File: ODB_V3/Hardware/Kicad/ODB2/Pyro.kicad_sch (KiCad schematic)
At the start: 51 parts, among them J1 Screw_Terminal_01x08, U11 SI5442DU-T1-GE3, U12 SI5442DU-T1-GE3, U2 LM339, U3 SI5442DU-T1-GE3, U8 SI5442DU-T1-GE3

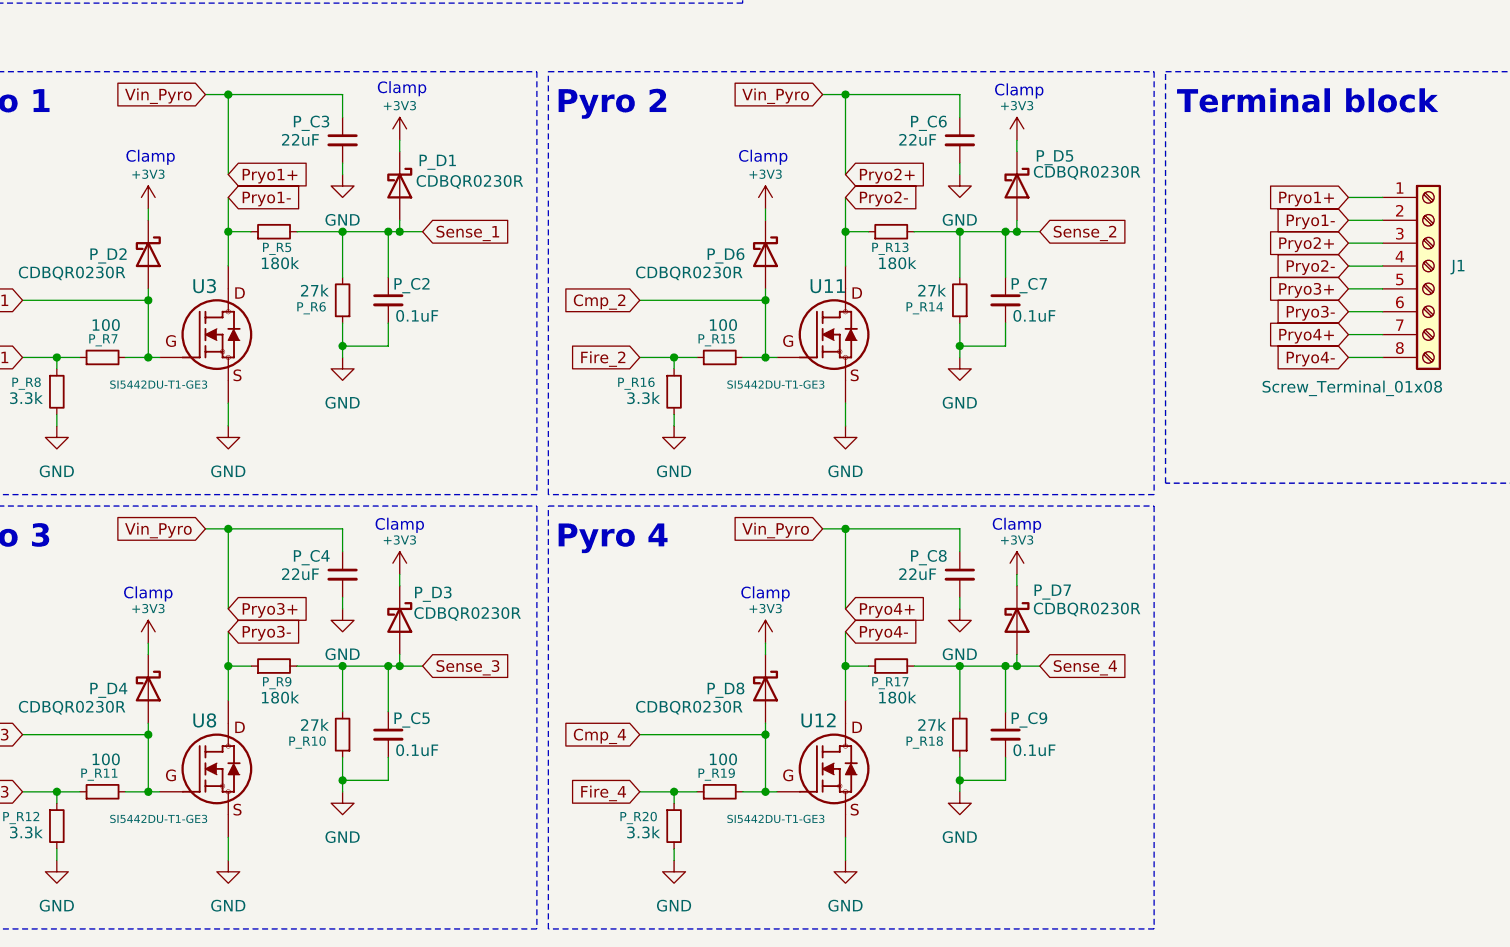
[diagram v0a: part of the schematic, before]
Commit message: wip: pyro trace
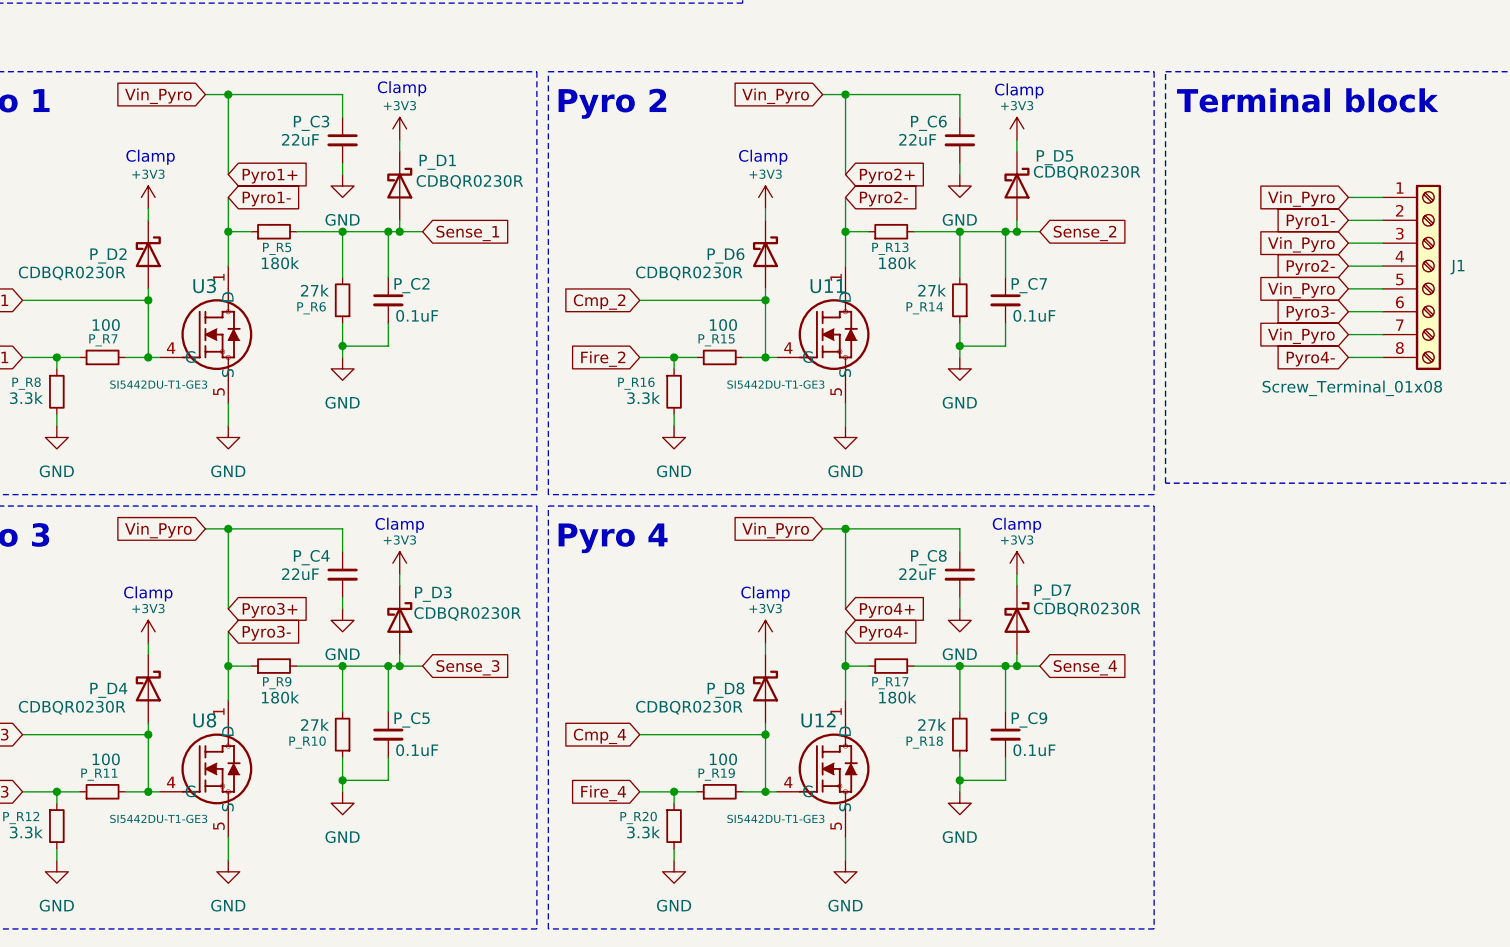
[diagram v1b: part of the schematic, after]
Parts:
- U11, U12, U3, U8: footprint ODB:SON_8DU-T1-GE3_VIS -> SON_8DU-T1-GE3_VIS
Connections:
- net Pryo1+ renamed Pyro1+
- net Pyro1+: now also PA_Q3.9 (D)
- net Pryo1- renamed Pyro1-
- net Pyro1-: now also U3.10 (D)
- net Pryo2- renamed Pyro2-
- net Pyro2-: now also U11.10 (D)
- net Pryo3- renamed Pyro3-
- net Pyro3-: now also U8.10 (D)
- net Pryo4- renamed Pyro4-
- net Pyro4-: now also U12.10 (D)
